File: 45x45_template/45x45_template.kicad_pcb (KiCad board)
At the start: 2 copper layers, 45 x 45 mm, 9 parts, among them J1 Screw_Terminal_01x02

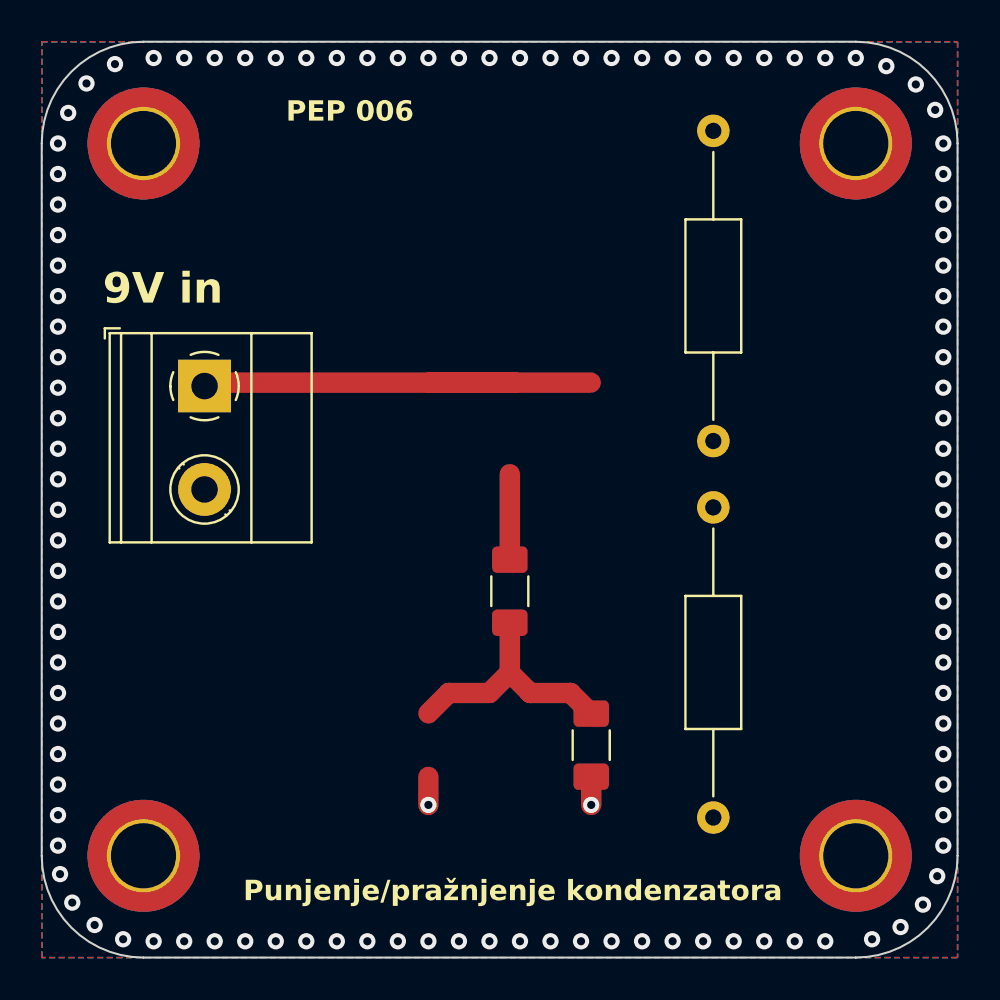
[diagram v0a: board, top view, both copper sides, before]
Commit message: Updated template.
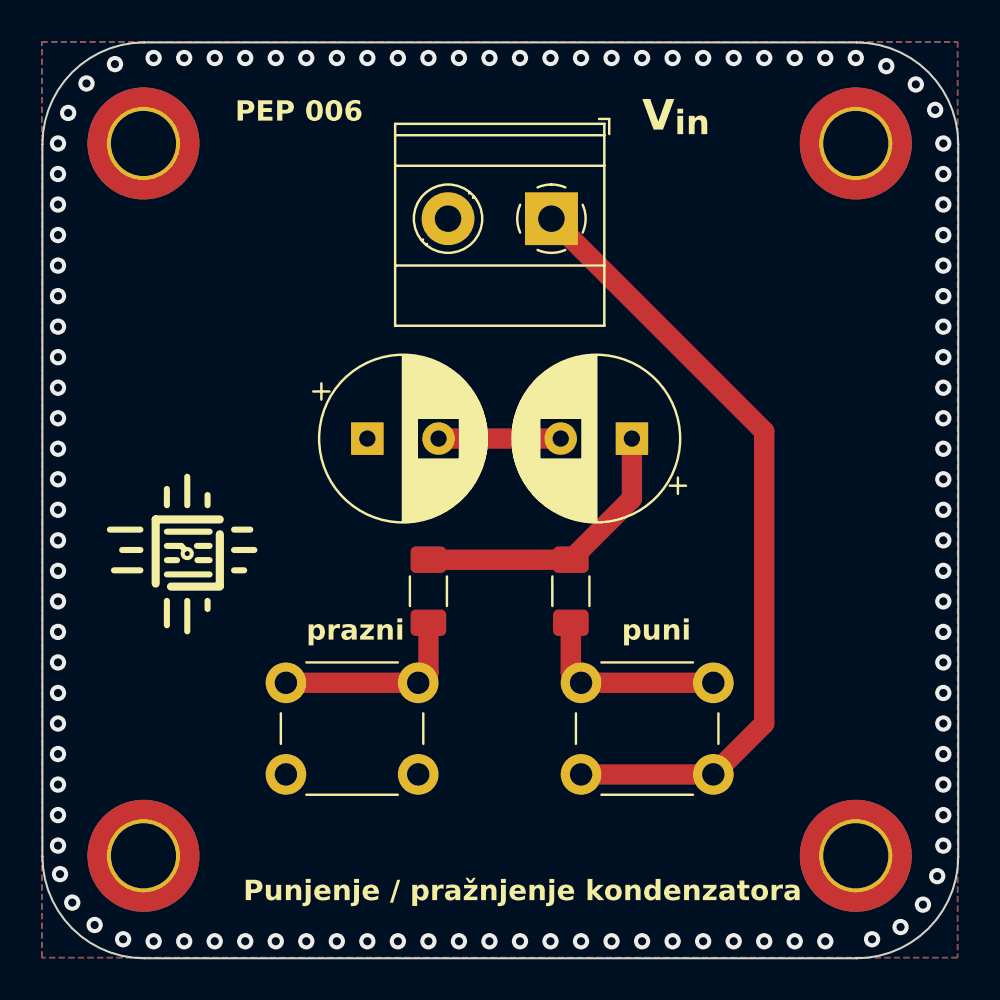
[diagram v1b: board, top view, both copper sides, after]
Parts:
- removed J1: Screw_Terminal_01x02, TerminalBlock_Phoenix:TerminalBlock_Phoenix_MKDS-1,5-2-5.08_1x02_P5.08mm_Horizontal
- removed R2: 100k, Resistor_SMD:R_1206_3216Metric_Pad1.30x1.75mm_HandSolder
- removed R3, R4: 100k, Resistor_THT:R_Axial_DIN0207_L6.3mm_D2.5mm_P15.24mm_Horizontal
- added C1: 100u, Capacitor_THT:CP_Radial_D8.0mm_P3.50mm, F.Cu at (133.0, 80.5)
- added C2: 100u, Capacitor_THT:CP_Radial_D8.0mm_P3.50mm, F.Cu at (120.0, 80.5)
- added J2: Screw_Terminal_01x02, TerminalBlock_Phoenix:TerminalBlock_Phoenix_MKDS-1,5-2-5.08_1x02_P5.08mm_Horizontal, F.Cu at (129.0, 69.7)
- added R6: 100k, Resistor_SMD:R_1206_3216Metric_Pad1.30x1.75mm_HandSolder, F.Cu at (123.0, 88.0)
- added REF**: ele_petnica_logo, PEP:ele_petnica_logo, F.Cu at (111.2, 86.2)
- added SW1: SW_Push, Button_Switch_THT:SW_PUSH_6mm_H4.3mm, F.Cu at (137.0, 97.0)
- added SW2: SW_Push, Button_Switch_THT:SW_PUSH_6mm_H4.3mm, F.Cu at (122.5, 97.0)
- moved R1 7.63 mm to (130.0, 88.0), turned to 90 degrees
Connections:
- R1 pad 1: out -> Net-(R1-Pad1)
- R1 pad 2: 0 -> Output voltage
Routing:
- net Input voltage: track 0.00 -> 39.2 mm
- net 9V: track 27.5 -> 0.00 mm
- net Output voltage: track 0.00 -> 14.2 mm
- net out: track 12.1 -> 0.00 mm
- net Net-(R6-Pad1): track 0.00 -> 9.66 mm
- net Net-(R1-Pad1): track 0.00 -> 9.66 mm
- net Net-(C1-Pad2): track 0.00 -> 6.00 mm
- net 0: track 2.76 -> 0.00 mm, vias 111 -> 109
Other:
- board text added: "Punjenje / pražnjenje kondenzatora"
- board text added: "V_{in}"
- board text added: "prazni"
- board text added: "puni"
- board text removed: "9V in"
- board text removed: "Punjenje/pražnjenje kondenzatora"
